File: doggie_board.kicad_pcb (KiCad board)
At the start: 2 copper layers, 127 x 127.5 mm, 40 parts, among them J1 XT90PW-M, Q1 PSMN3R7-100BSEJ, Q2 PSMN3R7-100BSEJ, Q3 PSMN3R7-100BSEJ, Q4 PSMN3R7-100BSEJ, Q5 PSMN3R7-100BSEJ, U1 TPS2490, U2 LM76005, U3 LM76005

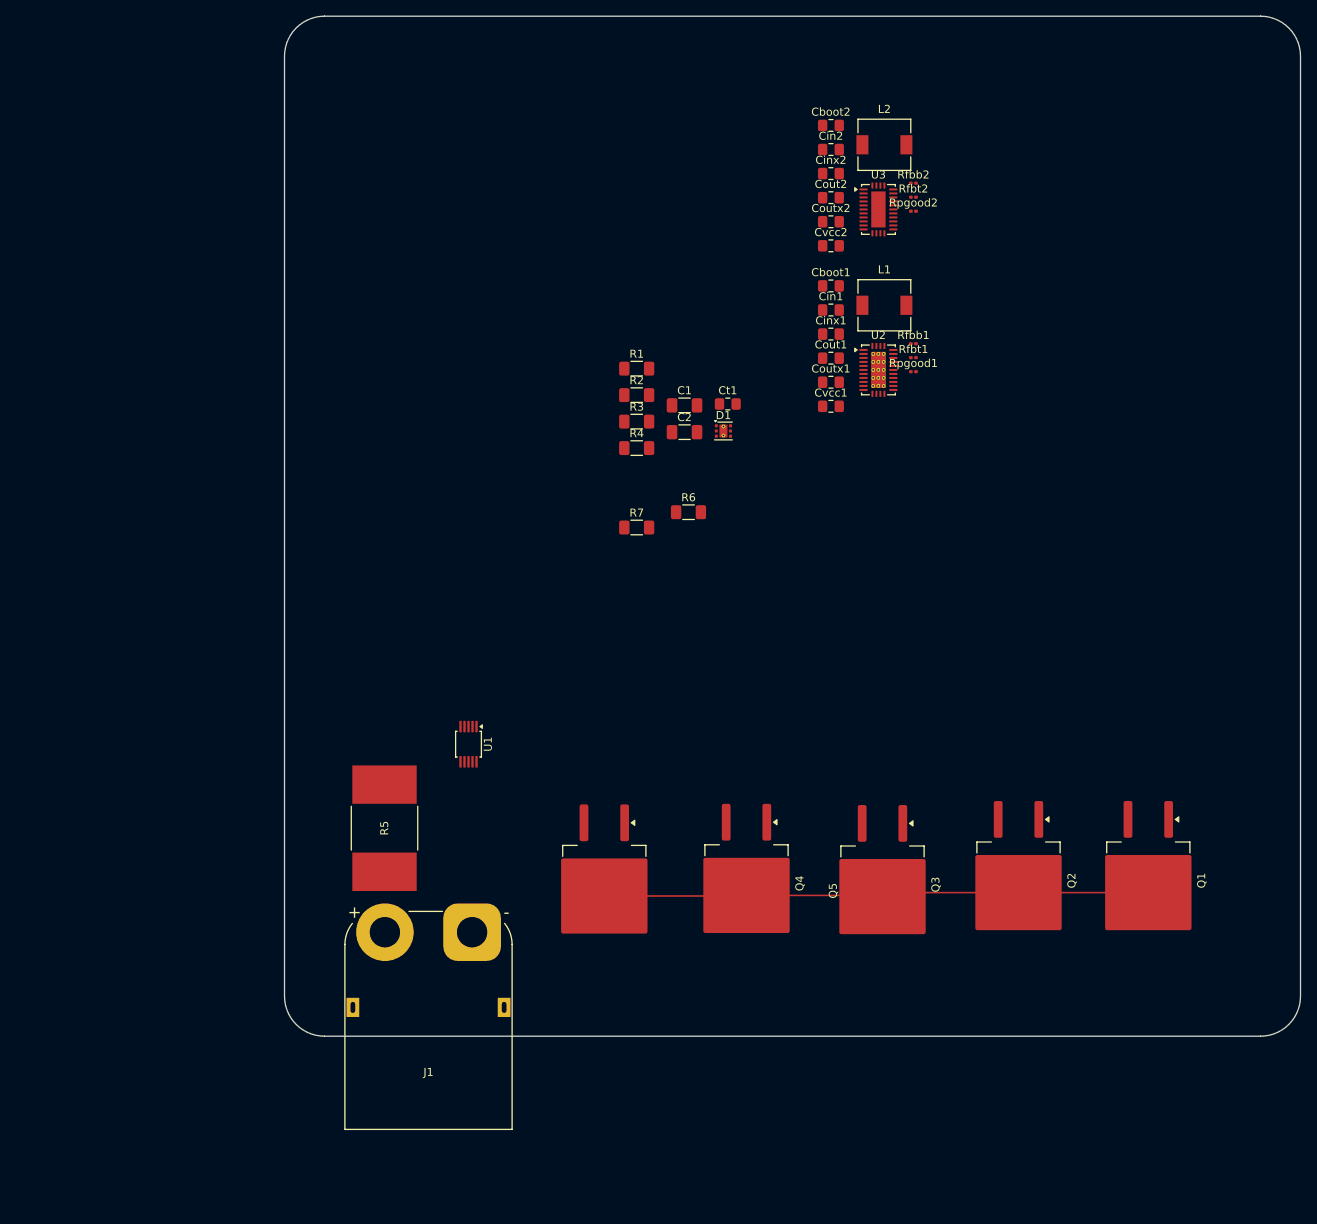
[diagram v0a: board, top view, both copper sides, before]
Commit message: updates
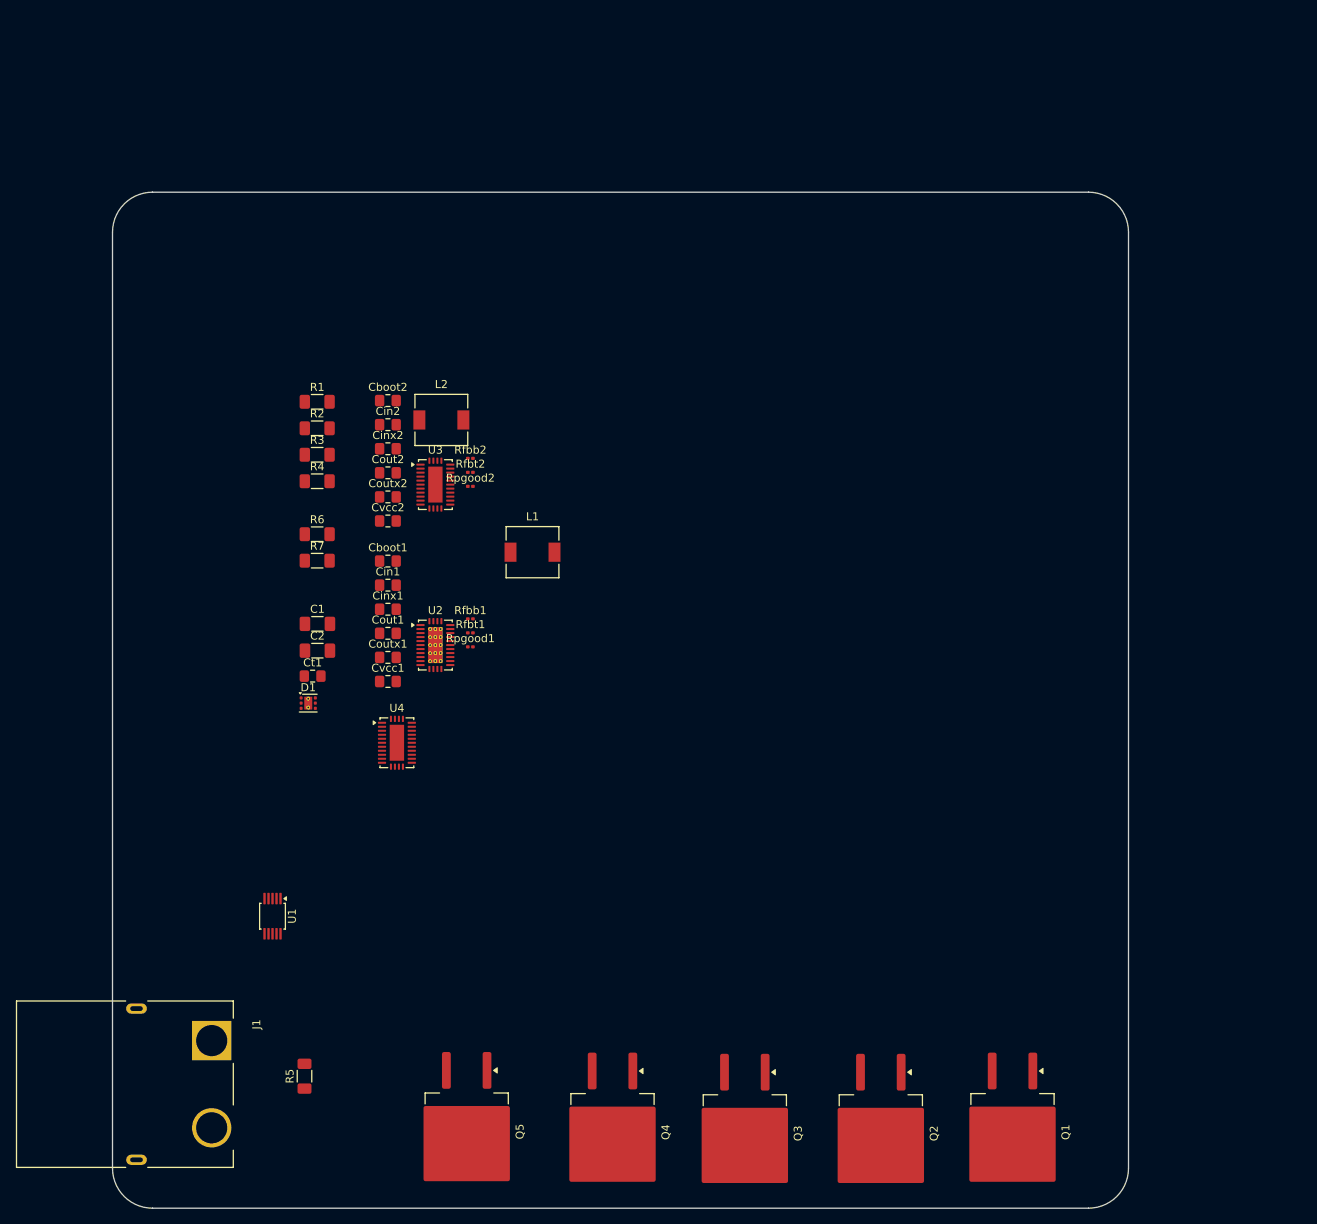
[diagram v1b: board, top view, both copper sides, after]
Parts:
- added U4: LM76005, Package_DFN_QFN:Texas_RNP0030B_WQFN-30-1EP_4x6mm_P0.5mm_EP1.8x4.5mm, F.Cu at (62.0, 109.3)
- J1: footprint Connector_AMASS:AMASS_XT90PW-M_1x02_P10.90mm_Horizontal -> vssop:AMASS_XT90PW-M
- R5: value 0.2mR, 15W -> 0.2m, 15W; footprint vssop:RES_PSR500_ROM -> Resistor_SMD:R_1206_3216Metric_Pad1.30x1.75mm_HandSolder
- moved Cboot1 65.2 mm to (60.9, 86.6)
- moved Cboot2 65.2 mm to (60.9, 66.5)
- moved Cin1 65.2 mm to (60.9, 89.6)
- moved Cin2 65.2 mm to (60.9, 69.6)
- moved Cinx1 65.2 mm to (60.9, 92.6)
- moved Cinx2 65.2 mm to (60.9, 72.6)
- moved Cout1 65.2 mm to (60.9, 95.6)
- moved Cout2 65.2 mm to (60.9, 75.6)
- moved Coutx1 65.2 mm to (60.9, 98.7)
- moved Coutx2 65.2 mm to (60.9, 78.6)
- moved Cvcc1 65.2 mm to (60.9, 101.7)
- moved Cvcc2 65.2 mm to (60.9, 81.6)
- moved L2 65.2 mm to (67.6, 69.0)
- moved Rfbb1 65.2 mm to (71.2, 93.8)
- moved Rfbb2 65.2 mm to (71.2, 73.8)
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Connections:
- Cin1 pad 1: V_switched -> 48v_switched
- Cin2 pad 1: V_switched -> 48v_switched
- Cinx1 pad 1: V_switched -> 48v_switched
- Cinx2 pad 1: V_switched -> 48v_switched
- Q1 pad 2: (no net) -> /High Side Power Switch/drain
- Q2 pad 2: (no net) -> /High Side Power Switch/drain
- Q3 pad 2: (no net) -> /High Side Power Switch/drain
- Q4 pad 2: (no net) -> /High Side Power Switch/drain
- Q5 pad 2: (no net) -> /High Side Power Switch/drain
- R5 pad 2: Net-(U1-SENSE) -> /High Side Power Switch/drain
- U1 pad 9: Net-(U1-SENSE) -> /High Side Power Switch/drain
- U2 pad 18: V_switched -> 48v_switched
- U2 pad 20: V_switched -> 48v_switched
- U2 pad 21: V_switched -> 48v_switched
- U2 pad 22: V_switched -> 48v_switched
- U3 pad 18: V_switched -> 48v_switched
- U3 pad 20: V_switched -> 48v_switched
- U3 pad 21: V_switched -> 48v_switched
- U3 pad 22: V_switched -> 48v_switched
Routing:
- net (no net): track 73.6 -> 0.00 mm
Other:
- board size 127 x 127.5 mm -> 127 x 127 mm
